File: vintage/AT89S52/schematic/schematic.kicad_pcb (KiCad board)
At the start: 2 copper layers, 64 x 120 mm, 15 parts, among them J1 P1, J2 P0, J3 P2, J4 P3, J5 ALE, J6 ~{PSEN}, J7 USB_A, SW1 Reset, U1 AT89S52, Y1 11.05920 MHz

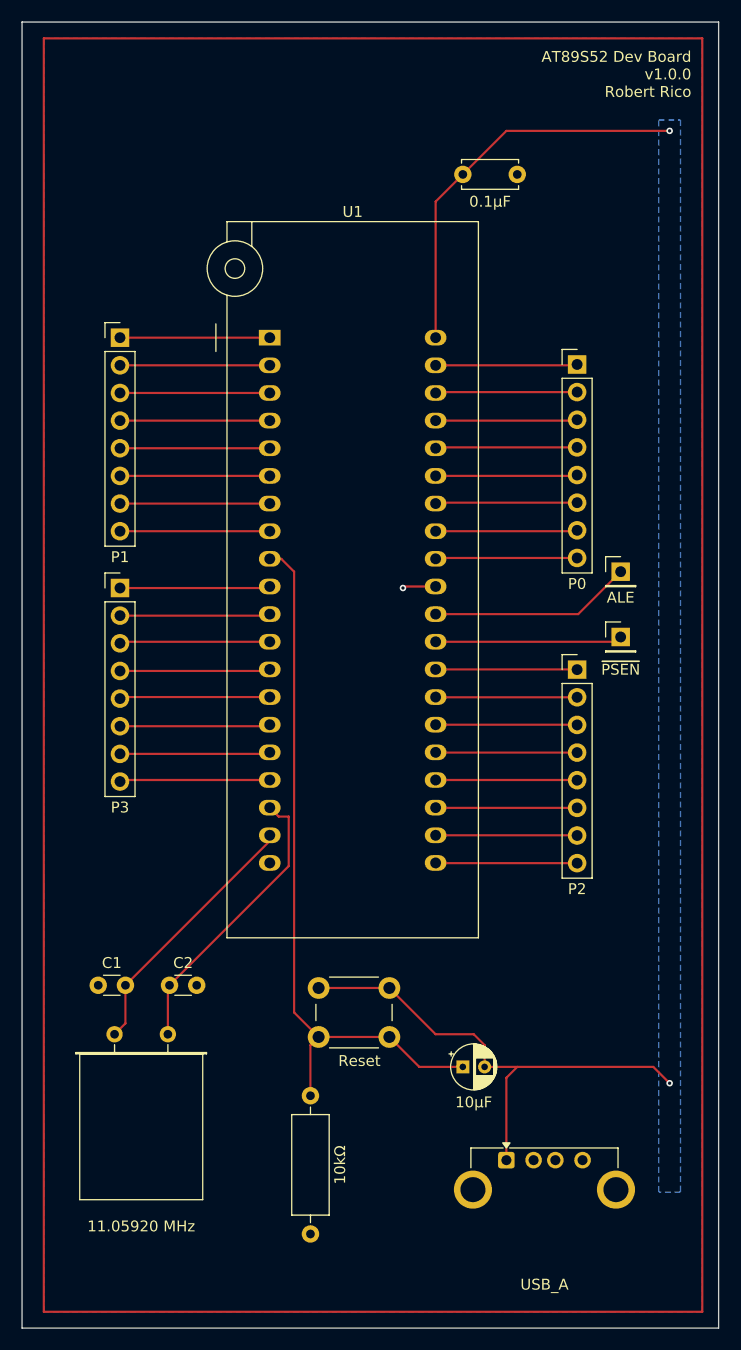
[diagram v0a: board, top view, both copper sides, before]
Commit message: AT89S52 Dev Board Fabrication Updates
Made some updates and fabrication file generation for Fabrication w/ JLCPCB
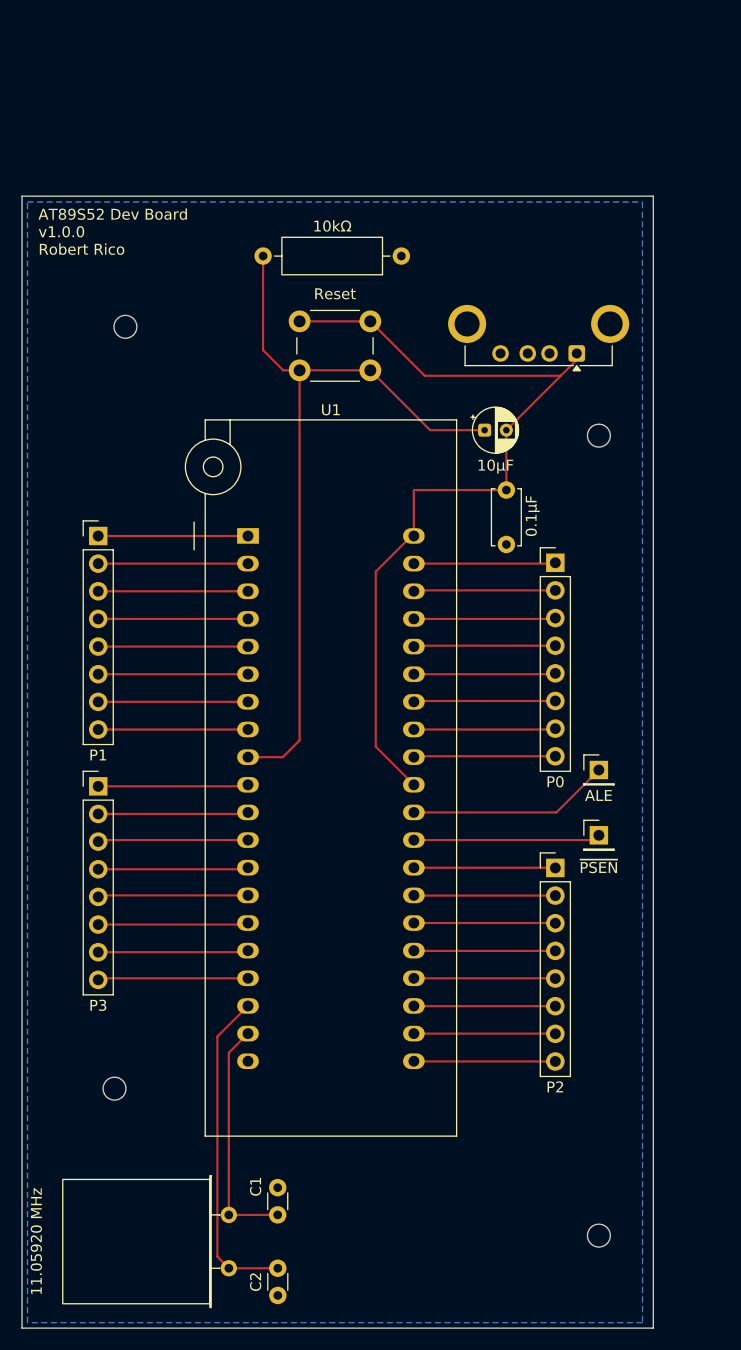
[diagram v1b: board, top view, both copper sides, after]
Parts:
- added REF**: MountingHole_2.1mm, MountingHole:MountingHole_2.1mm, F.Cu at (102.5, 127.5)
- added REF**: MountingHole_2.1mm, MountingHole:MountingHole_2.1mm, F.Cu at (58.0, 114.0)
- added REF**: MountingHole_2.1mm, MountingHole:MountingHole_2.1mm, F.Cu at (59.0, 44.0)
- added REF**: MountingHole_2.1mm, MountingHole:MountingHole_2.1mm, F.Cu at (102.5, 54.0)
- J7: value USB_A -> USB_B_Micro
- U1: footprint Socket:DIP_Socket-40_W11.9_W12.7_W15.24_W17.78_W18.5_3M_240-1280-00-0602J -> Socket:DIP_Socket-40_W11.9mm_W12.7mm_W15.24mm_W17.78mm_W18.5mm_3M_240-1280-00-0602J
- moved R1 90.2 mm to (84.3, 37.5), turned to 180 degrees
- moved J7 74.4 mm to (100.5, 46.4), turned to 180 degrees
- moved SW1 61.3 mm to (75.0, 43.5)
- moved C3 58.5 mm to (92.0, 53.5)
- moved C4 29.3 mm to (94.0, 59.0), turned to -90 degrees
- moved C2 27.8 mm to (73.0, 130.5), turned to -90 degrees
- moved C1 24.9 mm to (73.0, 123.1), turned to -90 degrees
- moved Y1 19.6 mm to (68.5, 125.6), turned to -90 degrees
- moved J2 18.3 mm to (98.5, 65.7)
- moved J1 18.3 mm to (56.5, 63.2)
- moved J3 18.3 mm to (98.5, 93.7)
- moved J4 18.3 mm to (56.5, 86.2)
- moved J5 18.3 mm to (102.5, 84.7)
- moved J6 18.3 mm to (102.5, 90.7)
- moved U1 18.3 mm to (70.3, 63.2)
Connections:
- J7 pad 4: GND -> unconnected-(J7-ID-Pad4)
- U1 pad 31: GND -> +5V
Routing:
- net Net-(U1-RST): track 66.5 -> 71.4 mm
- net Net-(U1-XTAL2): track 26.7 -> 30.2 mm
- net GND: track 3.06 -> 0.00 mm, vias 1 -> 0
- net +5V: track 82.7 -> 79.9 mm, vias 2 -> 0
- net Net-(U1-XTAL1): track 24.2 -> 22.4 mm
- removed copper zone on B.Cu, net +5V
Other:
- board size 64 x 120 mm -> 58 x 104 mm
